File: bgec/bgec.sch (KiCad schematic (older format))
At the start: 5 parts

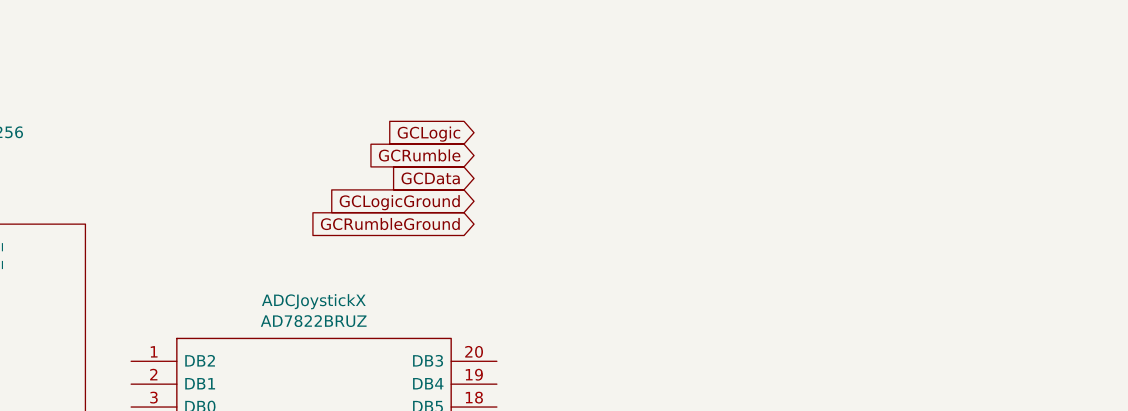
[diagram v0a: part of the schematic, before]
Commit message: Add clock
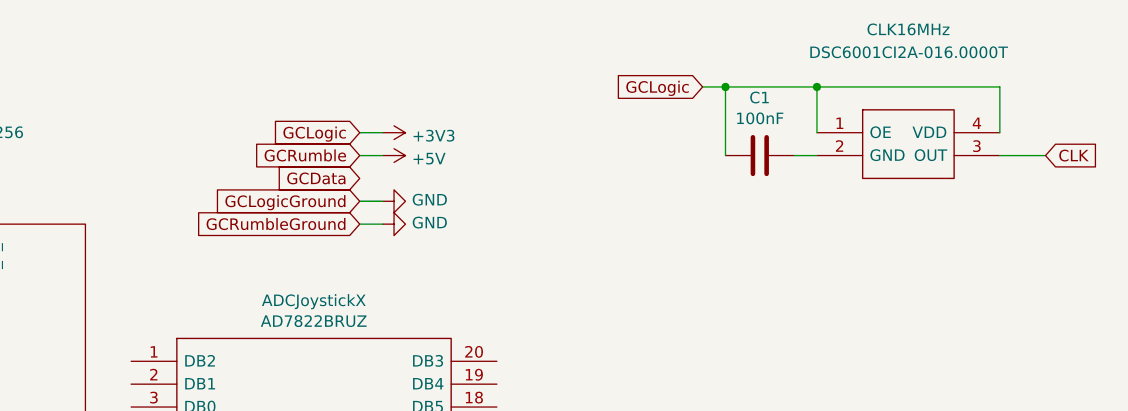
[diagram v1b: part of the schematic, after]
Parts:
- added C1: 100nF, symbol Device:C
- added CLK16MHz: DSC6001CI2A-016.0000T, 4-LEAD_CDFN-3.2X2.5_1, symbol bgec:DSC6001CI2A-016.0000T
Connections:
- net GCLogic renamed +3V3
- net +3V3: now also C1.1, CLK16MHz.1 (OE), CLK16MHz.4 (VDD)
- new net: C1.2, CLK16MHz.2 (GND)
- new net CLK: CLK16MHz.3 (OUT)
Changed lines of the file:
@@
 	1    0    0    -1
 $EndComp
-Text GLabel 6000 1000 0    50   Input ~ 0
+Text GLabel 5500 1000 0    50   Input ~ 0
 GCLogic
-Text GLabel 6000 1100 0    50   Input ~ 0
+Text GLabel 5500 1100 0    50   Input ~ 0
 GCRumble
-Text GLabel 6000 1200 0    50   Input ~ 0
+Text GLabel 5500 1200 0    50   Input ~ 0
 GCData
-Text GLabel 6000 1300 0    50   Input ~ 0
+Text GLabel 5500 1300 0    50   Input ~ 0
 GCLogicGround
-Text GLabel 6000 1400 0    50   Input ~ 0
+Text GLabel 5500 1400 0    50   Input ~ 0
 GCRumbleGround
 $Comp
@@
 	3900 1100 3900 1200
 Connection ~ 3800 1100
+$Comp
+L bgec:DSC6001CI2A-016.0000T CLK16MHz
+U 1 1 5E554F81
+P 7500 1000
+F 0 "CLK16MHz" H 7900 1450 50  0000 C CNN
+F 1 "DSC6001CI2A-016.0000T" H 7900 1350 50  0000 C CNN
+F 2 "4-LEAD_CDFN-3.2X2.5_1" H 8600 2500 50  0001 L CNN
+F 3 "https://componentsearchengine.com/Datasheets/1/DSC6001CI2A-016.0000T.pdf" H 8600 2400 50  0001 L CNN
+F 4 "Standard Clock Oscillators MEMS Oscillator, Ultra Low Power, LVCMOS, -40C-85C, 25ppm, 3.2x2.5mm" H 8600 2300 50  0001 L CNN "Description"
+F 5 "" H 8150 800 50  0001 L CNN "Height"
+F 6 "579-6001CI2A0160000T" H 8600 2100 50  0001 L CNN "Mouser Part Number"
+F 7 "https://www.mouser.com/Search/Refine.aspx?Keyword=579-6001CI2A0160000T" H 8600 2000 50  0001 L CNN "Mouser Price/Stock"
+F 8 "Microchip" H 8600 1900 50  0001 L CNN "Manufacturer_Name"
+F 9 "DSC6001CI2A-016.0000T" H 8600 1800 50  0001 L CNN "Manufacturer_Part_Number"
+	1    7500 1000
+	1    0    0    -1
+$EndComp
+Text GLabel 8500 1100 2    50   Input ~ 0
+CLK
+Wire Wire Line
+	8300 1100 8500 1100
+Text GLabel 7000 800  0    50   Input ~ 0
+GCLogic
+Wire Wire Line
+	8300 800  8300 1000
+Wire Wire Line
+	7500 1000 7500 800
+Connection ~ 7500 800
+Wire Wire Line
+	7500 800  8300 800
+Wire Wire Line
+	5500 1000 5600 1000
+$Comp
+L power:+3V3 #PWR?
+U 1 1 5E562812
+P 5600 1000
+F 0 "#PWR?" H 5600 850 50  0001 C CNN
+F 1 "+3V3" V 5615 1128 50  0000 L CNN
+F 2 "" H 5600 1000 50  0001 C CNN
+F 3 "" H 5600 1000 50  0001 C CNN
+	1    5600 1000
+	0    1    1    0
+$EndComp
+Wire Wire Line
+	5500 1100 5600 1100
+$Comp
+L power:+5V #PWR?
+U 1 1 5E564ED9
+P 5600 1100
+F 0 "#PWR?" H 5600 950 50  0001 C CNN
+F 1 "+5V" V 5615 1228 50  0000 L CNN
+F 2 "" H 5600 1100 50  0001 C CNN
+F 3 "" H 5600 1100 50  0001 C CNN
+	1    5600 1100
+	0    1    1    0
+$EndComp
+$Comp
+L Device:C C1
+U 1 1 5E566884
+P 7250 1100
+F 0 "C1" V 7502 1100 50  0000 C CNN
+F 1 "100nF" V 7411 1100 50  0000 C CNN
+F 2 "" H 7288 950 50  0001 C CNN
+F 3 "~" H 7250 1100 50  0001 C CNN
+	1    7250 1100
+	0    -1   -1   0
+$EndComp
+Wire Wire Line
+	7000 800  7100 800
+Wire Wire Line
+	7100 800  7100 1100
+Connection ~ 7100 800
+Wire Wire Line
+	7100 800  7500 800
+Wire Wire Line
+	7400 1100 7500 1100
+Wire Wire Line
+	5500 1300 5600 1300
+$Comp
+L power:GND #PWR?
+U 1 1 5E570CAB
+P 5600 1300
+F 0 "#PWR?" H 5600 1050 50  0001 C CNN
+F 1 "GND" V 5605 1172 50  0000 R CNN
+F 2 "" H 5600 1300 50  0001 C CNN
+F 3 "" H 5600 1300 50  0001 C CNN
+	1    5600 1300
+	0    -1   -1   0
+$EndComp
+$Comp
+L power:GND #PWR?
+U 1 1 5E5721CB
+P 5600 1400
+F 0 "#PWR?" H 5600 1150 50  0001 C CNN
+F 1 "GND" V 5605 1272 50  0000 R CNN
+F 2 "" H 5600 1400 50  0001 C CNN
+F 3 "" H 5600 1400 50  0001 C CNN
+	1    5600 1400
+	0    -1   -1   0
+$EndComp
+Wire Wire Line
+	5500 1400 5600 1400
 $EndSCHEMATC
